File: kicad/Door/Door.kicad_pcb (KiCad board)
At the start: 2 copper layers, 45.5 x 50.5 mm, 14 parts, among them Q1 NMOS, Q2 PMOS, SW1 Push Button, U1 NODEMCU v3

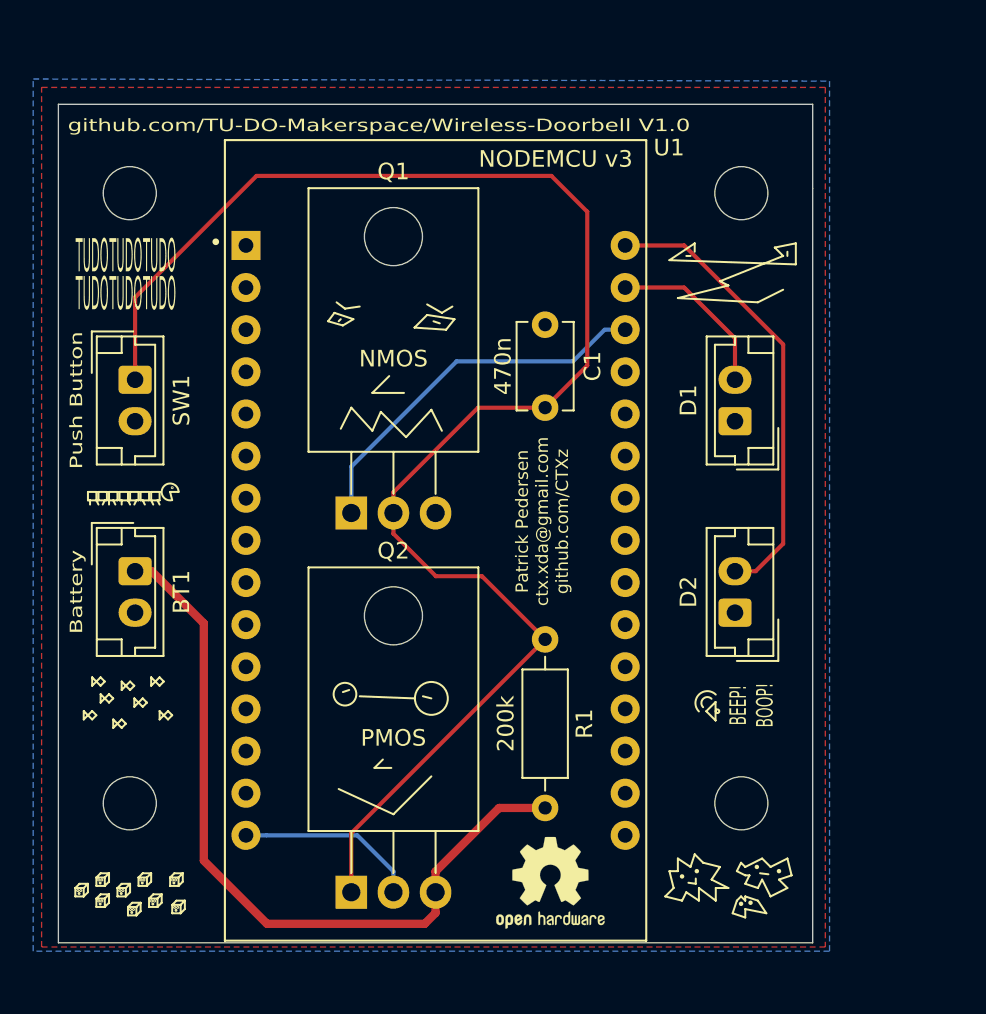
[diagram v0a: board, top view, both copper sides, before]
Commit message: Kicad: Finished 1st PCB revision
Signed-off-by: CTXz <ctx.xda@gmail.com>
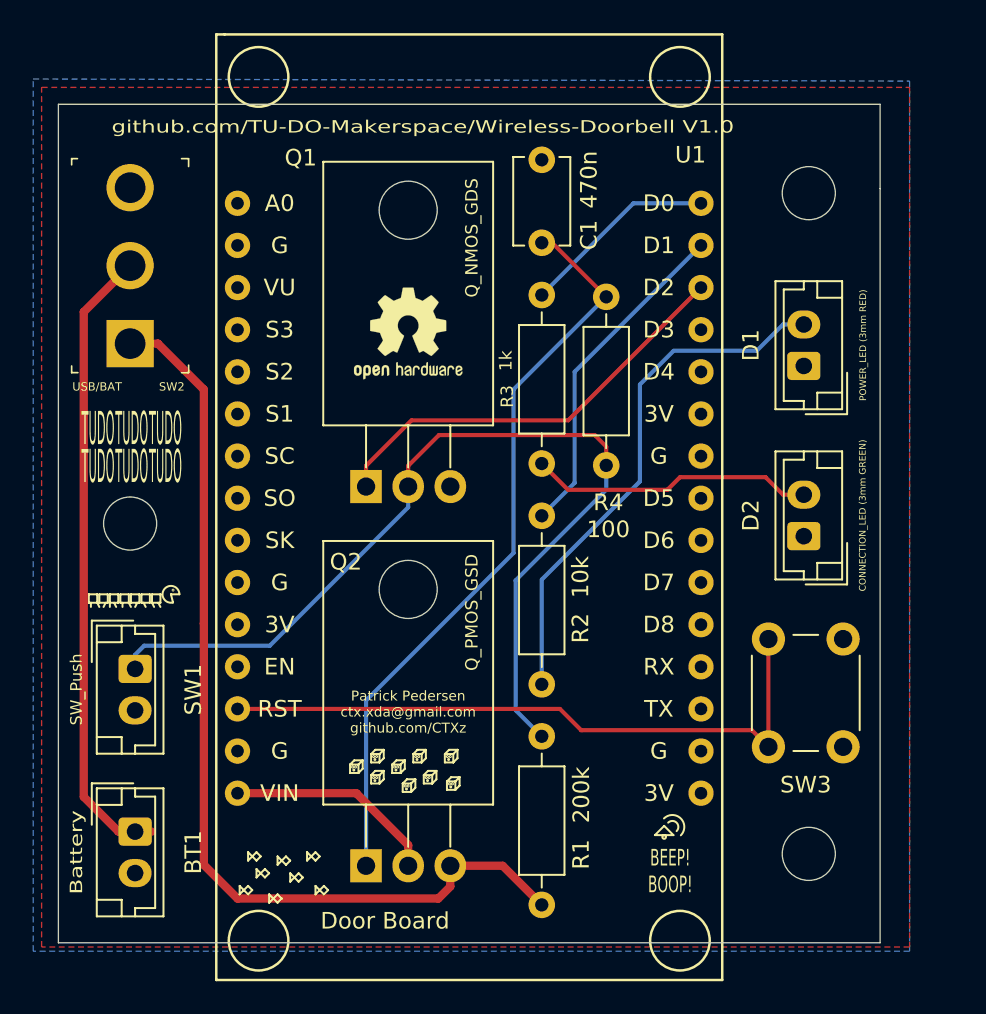
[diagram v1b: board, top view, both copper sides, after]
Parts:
- removed the REF** at (94.0, 131.8)
- removed the REF** at (57.1, 95.0)
- removed the REF** at (94.0, 95.0)
- added R2: 10k, Resistor_THT:R_Axial_DIN0207_L6.3mm_D2.5mm_P10.16mm_Horizontal, F.Cu at (82.0, 114.5)
- added R3: 1k, Resistor_THT:R_Axial_DIN0207_L6.3mm_D2.5mm_P10.16mm_Horizontal, F.Cu at (82.0, 101.2)
- added R4: 100, Resistor_THT:R_Axial_DIN0207_L6.3mm_D2.5mm_P10.16mm_Horizontal, F.Cu at (85.9, 111.4)
- added REF**: MountingHole_3.2mm_M3, MountingHole:MountingHole_3.2mm_M3, F.Cu at (98.1, 95.0)
- added REF**: MountingHole_3.2mm_M3, MountingHole:MountingHole_3.2mm_M3, F.Cu at (98.1, 134.8)
- added SW2: USB/BAT, digikey-footprints:Toggle_Switch_100SP1T1B4M2QE, F.Cu at (57.2, 104.1)
- added SW3: RST_BTN, Button_Switch_THT:SW_PUSH_6mm, F.Cu at (95.6, 128.4)
- D1: value POWER_LED -> POWER_LED (3mm RED)
- D2: value CONNECTION_LED -> CONNECTION_LED (3mm GREEN)
- Q1: value NMOS -> Q_NMOS_GDS
- Q2: value PMOS -> Q_PMOS_GSD
- SW1: value Push Button -> SW_Push
- U1: footprint ZC563900_FP:MODULE_ZC563900 -> ESP8266-Kicad:NodeMCU-LoLinV3
- moved REF** 34.2 mm to (73.9, 103.5)
- moved SW1 17.4 mm to (57.5, 123.7)
- moved REF** 16.9 mm to (57.2, 114.9)
- moved BT1 15.7 mm to (57.5, 133.5)
- moved C1 9.94 mm to (82.0, 98.0)
- moved D2 6.20 mm to (97.8, 115.7)
- moved R1 5.85 mm to (82.0, 127.8)
- moved D1 5.32 mm to (97.8, 105.4)
- moved U1 2.03 mm to (77.6, 116.0)
- moved Q1 1.82 mm to (71.4, 112.7)
- moved Q2 1.82 mm to (71.4, 135.6)
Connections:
- net Net-(U1-Pad27) renamed DBG_BTN
- BT1 pad 1: 9V_BAT_+ -> Net-(BT1-Pad1)
- D1 pad 2: POWER_LED -> Net-(D1-Pad2)
- D2 pad 2: CONNECTION_LED -> Net-(D2-Pad2)
- Q1 pad 2: Net-(C1-Pad1) -> Net-(Q1-Pad2)
- R1 pad 1: Net-(C1-Pad1) -> Net-(Q1-Pad2)
- SW1 pad 1: Net-(C1-Pad1) -> Net-(Q1-Pad2)
- U1 pad 11: Net-(U1-Pad11) -> (no net)
- U1 pad 13: Net-(U1-Pad13) -> RST_BTN
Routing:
- net Net-(Q1-Pad2): track 0.00 -> 56.9 mm
- net Net-(C1-Pad1): track 94.6 -> 45.5 mm
- net RST_BTN: track 0.00 -> 39.5 mm
- net Net-(BT1-Pad1): track 0.00 -> 38.1 mm
- net Net-(D1-Pad2): track 0.00 -> 31.9 mm
- net Net-(D2-Pad2): track 0.00 -> 17.2 mm
- net CONNECTION_LED: track 27.6 -> 11.9 mm
- net 9V_BAT_+: track 46.3 -> 58.0 mm
- net POWER_LED: track 10.4 -> 20.3 mm
- net POWER_LATCH: track 22.7 -> 25.9 mm
- net NODE_VIN: track 11.0 -> 12.8 mm
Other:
- board size 45.5 x 50.5 mm -> 49.5 x 50.5 mm
- board text added: "Door Board"

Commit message: Kicad: Updated to v6.0
Signed-off-by: Patrick Pedersen <ctx.xda@gmail.com>
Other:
- net class Default removed
